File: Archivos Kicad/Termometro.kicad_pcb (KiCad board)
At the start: 2 copper layers, 53.3 x 67.8 mm, 22 parts, among them SW1 SW_Push, SW2 SW_Push, SW3 SW_Push, SW4 SW_Push, U1 LM358, U2 CC56-12EWA

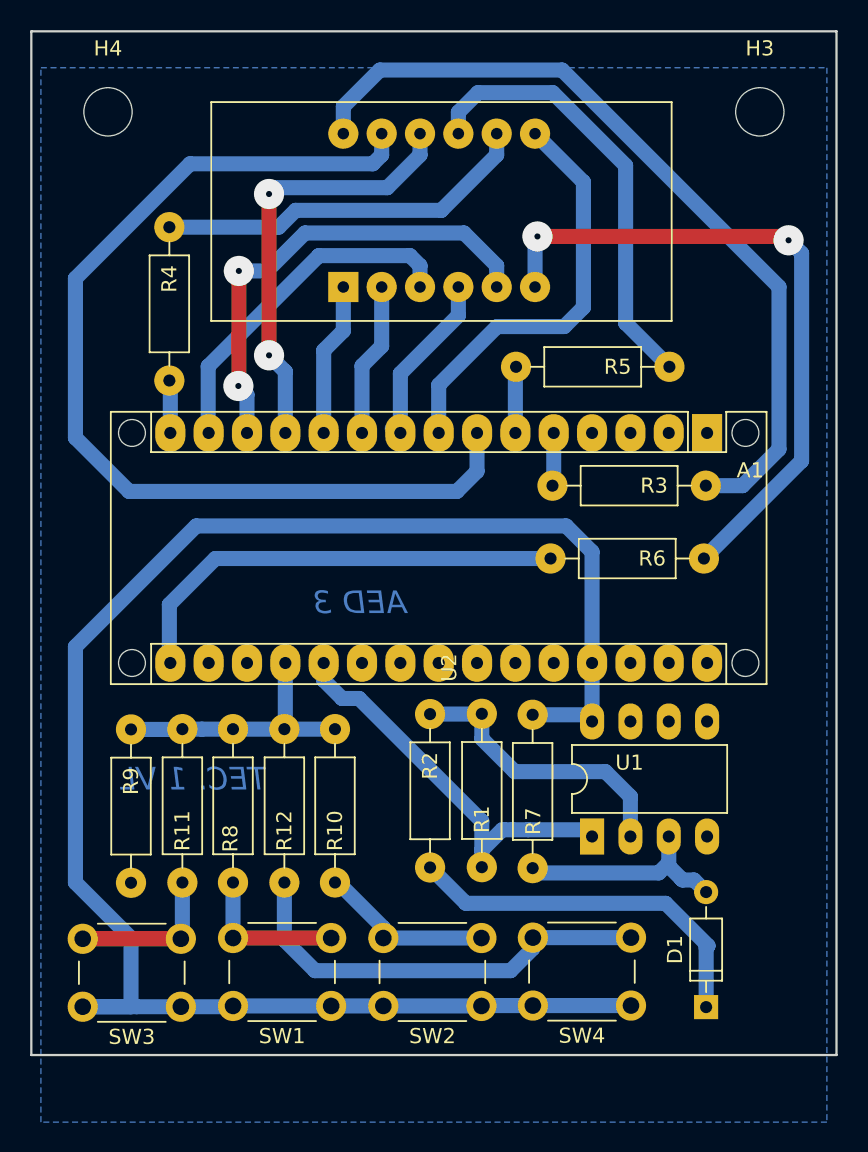
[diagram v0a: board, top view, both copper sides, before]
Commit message: correccion del board
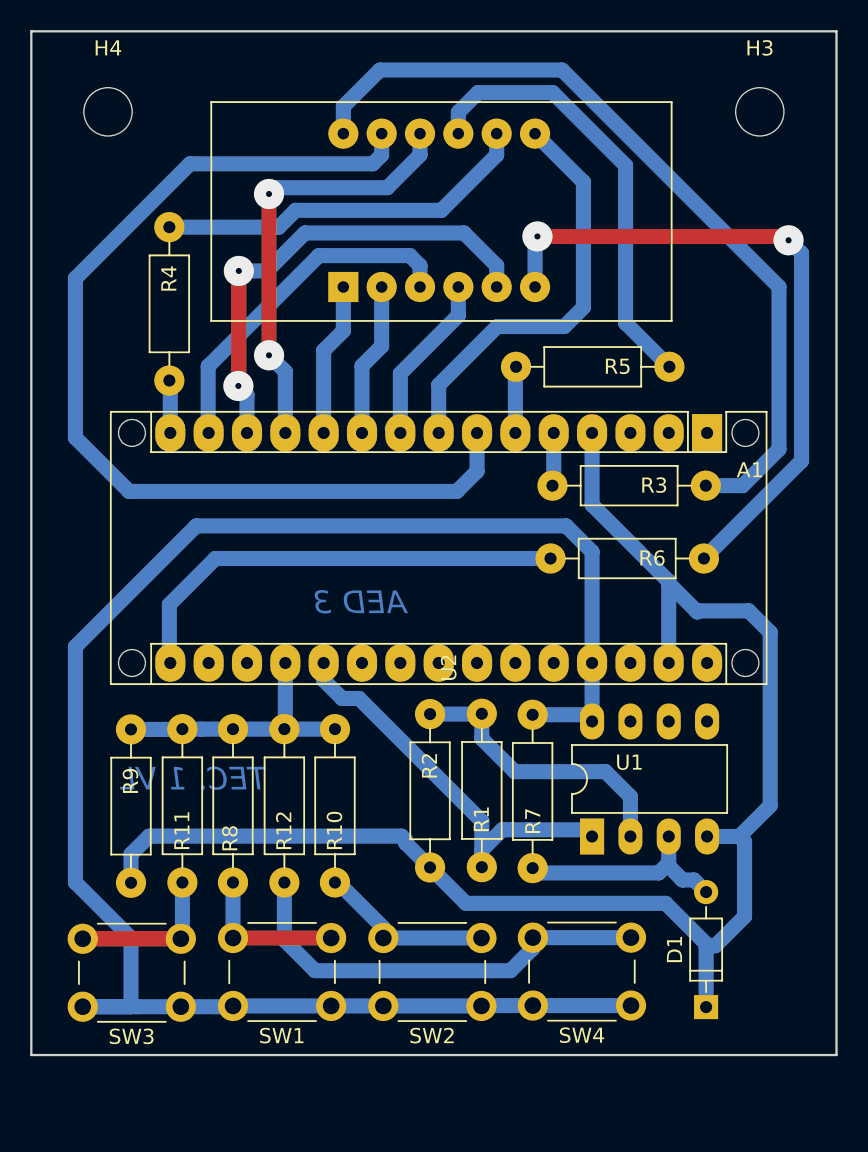
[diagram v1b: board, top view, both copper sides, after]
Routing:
- net GND: track 24.7 -> 98.6 mm
- removed copper zone on B.Cu, net GND
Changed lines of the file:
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@@
   (segment (start 136.673165 116.343767) (end 140.082165 116.343767) (width 1) (layer "B.Cu") (net 1))
   (segment (start 142.283665 120.156267) (end 140.102165 117.974767) (width 1) (layer "B.Cu") (net 1))
+  (segment (start 159.204186 110.926788) (end 157.782165 109.504767) (width 1) (layer "B.Cu") (net 2))
+  (segment (start 116.861165 125.625767) (end 118.057165 124.429767) (width 1) (layer "B.Cu") (net 2))
+  (segment (start 154.382165 109.579767) (end 152.484665 107.682267) (width 1) (layer "B.Cu") (net 2))
+  (segment (start 152.484665 107.682267) (end 152.484665 107.557267) (width 1) (layer "B.Cu") (net 2))
+  (segment (start 147.404665 97.718267) (end 147.404665 102.477267) (width 1) (layer "B.Cu") (net 2))
+  (segment (start 118.057165 124.429767) (end 134.782165 124.429767) (width 1) (layer "B.Cu") (net 2))
+  (segment (start 154.457165 109.504767) (end 154.382165 109.579767) (width 1) (layer "B.Cu") (net 2))
+  (segment (start 157.782165 109.504767) (end 154.457165 109.504767) (width 1) (layer "B.Cu") (net 2))
+  (segment (start 155.024665 124.451767) (end 157.160165 124.451767) (width 1) (layer "B.Cu") (net 2))
+  (segment (start 155.088165 131.690767) (end 155.571165 131.690767) (width 1) (layer "B.Cu") (net 2))
   (segment (start 154.961165 131.817767) (end 154.961165 135.754767) (width 1) (layer "B.Cu") (net 2))
+  (segment (start 159.204186 122.407746) (end 159.204186 110.926788) (width 1) (layer "B.Cu") (net 2))
   (segment (start 139.049548 128.88015) (end 152.277548 128.88015) (width 1) (layer "B.Cu") (net 2))
+  (segment (start 135.057165 124.704767) (end 135.057165 124.887767) (width 1) (layer "B.Cu") (net 2))
   (segment (start 136.673165 126.503767) (end 139.049548 128.88015) (width 1) (layer "B.Cu") (net 2))
+  (segment (start 157.507165 124.798767) (end 157.160165 124.451767) (width 1) (layer "B.Cu") (net 2))
+  (segment (start 147.404665 102.477267) (end 152.484665 107.557267) (width 1) (layer "B.Cu") (net 2))
+  (segment (start 157.507165 129.754767) (end 157.507165 124.798767) (width 1) (layer "B.Cu") (net 2))
+  (segment (start 116.861165 127.519767) (end 116.861165 125.625767) (width 1) (layer "B.Cu") (net 2))
   (segment (start 155.088165 131.690767) (end 154.961165 131.817767) (width 1) (layer "B.Cu") (net 2))
+  (segment (start 157.160165 124.451767) (end 159.204186 122.407746) (width 1) (layer "B.Cu") (net 2))
+  (segment (start 135.057165 124.887767) (end 136.673165 126.503767) (width 1) (layer "B.Cu") (net 2))
+  (segment (start 155.571165 131.690767) (end 157.507165 129.754767) (width 1) (layer "B.Cu") (net 2))
   (segment (start 152.277548 128.88015) (end 155.088165 131.690767) (width 1) (layer "B.Cu") (net 2))
+  (segment (start 134.782165 124.429767) (end 135.057165 124.704767) (width 1) (layer "B.Cu") (net 2))
+  (segment (start 152.484665 107.557267) (end 152.484665 112.958267) (width 1) (layer "B.Cu") (net 2))
   (segment (start 154.941165 101.210767) (end 157.374165 101.210767) (width 1) (layer "B.Cu") (net 3))
   (segment (start 159.787165 98.797767) (end 159.787165 88.041139) (width 1) (layer "B.Cu") (net 3))
@@
   (segment (start 116.861165 117.359767) (end 120.244765 117.359767) (width 1) (layer "B.Cu") (net 38))
   (segment (start 117.242165 117.339767) (end 117.242165 117.212767) (width 1) (layer "B.Cu") (net 38))
-  (zone (net 2) (net_name "GND") (layer "B.Cu") (hatch edge 0.508)
-    (connect_pads (clearance 1.5))
-    (min_thickness 0.254) (filled_areas_thickness no)
-    (fill yes (thermal_gap 0.5) (thermal_bridge_width 0.5) (smoothing chamfer) (radius 0.7))
-    (polygon
-      (pts
-        (xy 162.962165 143.374767)
-        (xy 110.892165 143.374767)
-        (xy 110.892165 73.524767)
-        (xy 162.962165 73.524767)
-      )
-    )
-  )
 )
